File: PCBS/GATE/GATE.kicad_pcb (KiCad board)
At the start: 2 copper layers, 29 x 14 mm, 14 parts, among them J1 Conn_01x01_Socket, J2 Conn_01x01_Socket, J3 Conn_01x03_Socket, U1 SN74LVC1G32DBVR

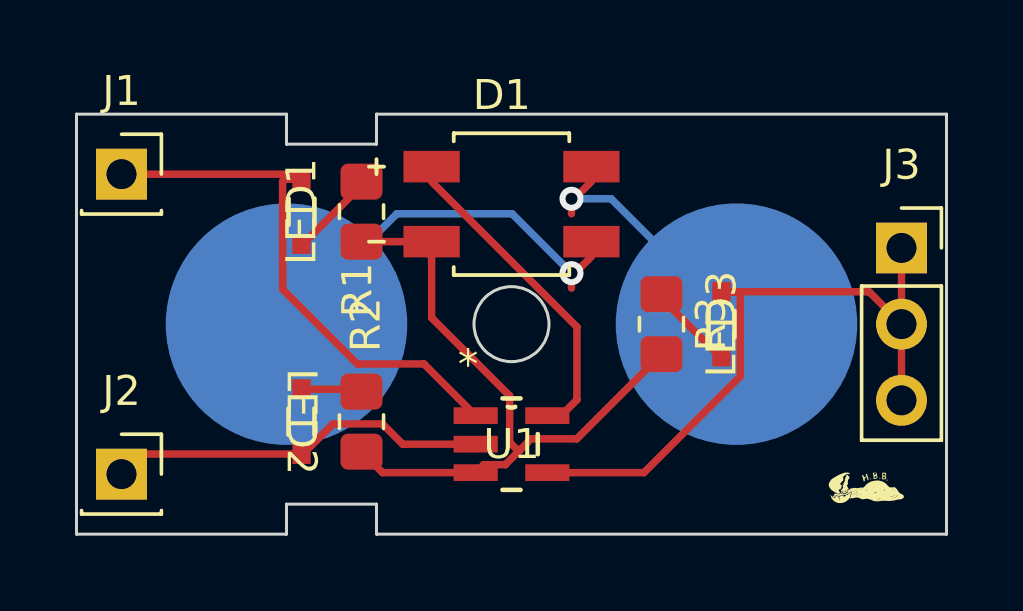
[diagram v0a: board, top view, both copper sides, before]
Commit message: Added Board PCB
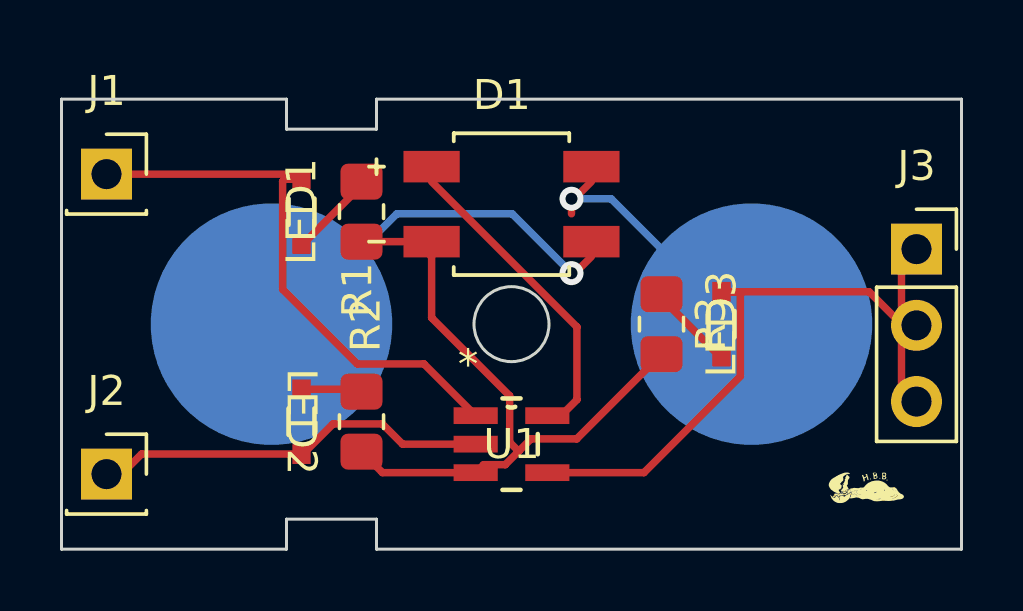
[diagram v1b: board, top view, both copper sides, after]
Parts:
- moved J3 0.50 mm to (168.5, 85.0)
- moved J1 0.50 mm to (141.5, 82.5)
- moved J2 0.50 mm to (141.5, 92.5)
- moved J4 0.50 mm to (147.0, 87.5)
- moved J5 0.50 mm to (163.0, 87.5)
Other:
- board size 29 x 14 mm -> 30 x 15 mm
- board text added: "GATE PCB REV 1"
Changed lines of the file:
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@@
       (outputformat 1)
       (mirror false)
-      (drillshape 1)
+      (drillshape 0)
       (scaleselection 1)
-      (outputdirectory "")
+      (outputdirectory "production/Rev1/")
     )
   )
@@
     (fp_line (start 1 0.625) (end -1 0.625)
       (stroke (width 0.1) (type solid)) (layer "F.Fab"))
-    (pad "1" smd roundrect locked (at -1 0 270) (size 1.2 1.4) (layers "F.Cu" "F.Paste" "F.Mask") (roundrect_rratio 0.208333)
+    (pad "1" smd roundrect locked (at -1 0 270) (size 1.2 1.4) (layers "F.Cu" "F.Paste" "F.Mask") (roundrect_rratio 0.2083333333)
       (net 5 "Net-(LED3-Pad1)") (pintype "passive"))
-    (pad "2" smd roundrect locked (at 1 0 270) (size 1.2 1.4) (layers "F.Cu" "F.Paste" "F.Mask") (roundrect_rratio 0.208333)
+    (pad "2" smd roundrect locked (at 1 0 270) (size 1.2 1.4) (layers "F.Cu" "F.Paste" "F.Mask") (roundrect_rratio 0.2083333333)
       (net 1 "GND") (pintype "passive"))
     (model "${KICAD6_3DMODEL_DIR}/Resistor_SMD.3dshapes/R_0805_2012Metric.wrl"
@@
     (fp_line (start 1 0.625) (end -1 0.625)
       (stroke (width 0.1) (type solid)) (layer "F.Fab"))
-    (pad "1" smd roundrect (at -1 0 270) (size 1.2 1.4) (layers "F.Cu" "F.Paste" "F.Mask") (roundrect_rratio 0.208333)
+    (pad "1" smd roundrect (at -1 0 270) (size 1.2 1.4) (layers "F.Cu" "F.Paste" "F.Mask") (roundrect_rratio 0.2083333333)
       (net 3 "Net-(LED1-Pad1)") (pintype "passive"))
-    (pad "2" smd roundrect (at 1 0 270) (size 1.2 1.4) (layers "F.Cu" "F.Paste" "F.Mask") (roundrect_rratio 0.208333)
+    (pad "2" smd roundrect (at 1 0 270) (size 1.2 1.4) (layers "F.Cu" "F.Paste" "F.Mask") (roundrect_rratio 0.2083333333)
       (net 1 "GND") (pintype "passive"))
     (model "${KICAD6_3DMODEL_DIR}/Resistor_SMD.3dshapes/R_0805_2012Metric.wrl"
@@
     (fp_line (start 1 0.625) (end -1 0.625)
       (stroke (width 0.1) (type solid)) (layer "F.Fab"))
-    (pad "1" smd roundrect (at -1 0 270) (size 1.2 1.4) (layers "F.Cu" "F.Paste" "F.Mask") (roundrect_rratio 0.208333)
+    (pad "1" smd roundrect (at -1 0 270) (size 1.2 1.4) (layers "F.Cu" "F.Paste" "F.Mask") (roundrect_rratio 0.2083333333)
       (net 4 "Net-(LED2-Pad1)") (pintype "passive"))
-    (pad "2" smd roundrect (at 1 0 270) (size 1.2 1.4) (layers "F.Cu" "F.Paste" "F.Mask") (roundrect_rratio 0.208333)
+    (pad "2" smd roundrect (at 1 0 270) (size 1.2 1.4) (layers "F.Cu" "F.Paste" "F.Mask") (roundrect_rratio 0.2083333333)
       (net 1 "GND") (pintype "passive"))
     (model "${KICAD6_3DMODEL_DIR}/Resistor_SMD.3dshapes/R_0805_2012Metric.wrl"
@@
   )
   (footprint "Connector_PinSocket_2.54mm:PinSocket_1x01_P2.54mm_Vertical" (layer "F.Cu")
-    (at 142 82.5)
+    (at 141.5 82.5)
     (descr "Through hole straight socket strip, 1x01, 2.54mm pitch, single row (from Kicad 4.0.7), script generated")
     (tags "Through hole socket strip THT 1x01 2.54mm single row")
@@
   )
   (footprint "Connector_PinSocket_2.54mm:PinSocket_1x01_P2.54mm_Vertical" (layer "F.Cu")
-    (at 142 92.5)
+    (at 141.5 92.5)
     (descr "Through hole straight socket strip, 1x01, 2.54mm pitch, single row (from Kicad 4.0.7), script generated")
     (tags "Through hole socket strip THT 1x01 2.54mm single row")
@@
   )
   (footprint "Connector_PinSocket_2.54mm:PinSocket_1x03_P2.54mm_Vertical" (layer "F.Cu")
-    (at 168 84.96)
+    (at 168.5 85)
     (descr "Through hole straight socket strip, 1x03, 2.54mm pitch, single row (from Kicad 4.0.7), script generated")
     (tags "Through hole socket strip THT 1x03 2.54mm single row")
@@
   )
   (footprint "DigitalLogicFootprints:8mm-snap" locked (layer "B.Cu")
-    (at 147.5 87.5 180)
+    (at 147 87.5 180)
     (property "Sheetfile" "ANDGATE.kicad_sch")
     (property "Sheetname" "")
@@
   )
   (footprint "DigitalLogicFootprints:8mm-snap" locked (layer "B.Cu")
-    (at 162.5 87.5 180)
+    (at 163 87.5 180)
     (property "Sheetfile" "ANDGATE.kicad_sch")
     (property "Sheetname" "")
@@
   (gr_poly
     (pts
-      (xy 140.5 80.5)
-      (xy 147.5 80.5)
-      (xy 147.5 81.5)
-      (xy 150.5 81.5)
-      (xy 150.5 80.5)
-      (xy 169.5 80.5)
-      (xy 169.5 94.5)
-      (xy 150.5 94.5)
-      (xy 150.5 93.5)
-      (xy 147.5 93.5)
-      (xy 147.5 94.5)
-      (xy 140.5 94.5)
+      (xy 140 95)
+      (xy 140 80)
+      (xy 147.5 80)
+      (xy 147.5 81)
+      (xy 150.5 81)
+      (xy 150.5 80)
+      (xy 170 80)
+      (xy 170 95)
+      (xy 150.5 95)
+      (xy 150.5 94)
+      (xy 147.5 94)
+      (xy 147.5 95)
     )
     (stroke (width 0.1) (type solid)) (fill none) (layer "Edge.Cuts"))
-  (gr_circle (center 165.1 81.28) (end 165.1 81.28)
-    (stroke (width 0.1) (type default)) (fill none) (layer "Edge.Cuts"))
   (gr_circle (center 155 87.5) (end 156.25 87.5)
     (stroke (width 0.1) (type default)) (fill none) (layer "Edge.Cuts"))
+  (gr_text "GATE PCB REV 1" (at 165 82) (layer "B.SilkS")
+    (effects (font (size 1 1) (thickness 0.15)) (justify left bottom mirror))
+  )
   (segment (start 155.653749 91.324052) (end 157.175948 91.324052) (width 0.25) (layer "F.Cu") (net 1))
   (segment (start 150.700001 92.450001) (end 153.8062 92.450001) (width 0.25) (layer "F.Cu") (net 1))
@@
   (segment (start 157 83.32) (end 158.32 83.32) (width 0.25) (layer "B.Cu") (net 9))
   (segment (start 158.32 83.32) (end 162.5 87.5) (width 0.25) (layer "B.Cu") (net 9))
-  (segment (start 157 86.3) (end 157 85.9125) (width 0.25) (layer "F.Cu") (net 10))
   (segment (start 157 85.9125) (end 157.6625 85.25) (width 0.25) (layer "F.Cu") (net 10))
   (via (at 157 85.8) (size 0.8) (drill 0.4) (layers "F.Cu" "B.Cu") (net 10))
